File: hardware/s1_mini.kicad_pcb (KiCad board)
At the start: 2 copper layers, 31 x 54.4 mm, 12 parts, among them P1 USB_Edge, U1 AP2114H, U2 SM220UF1, U3 Wemos_D1_Mini

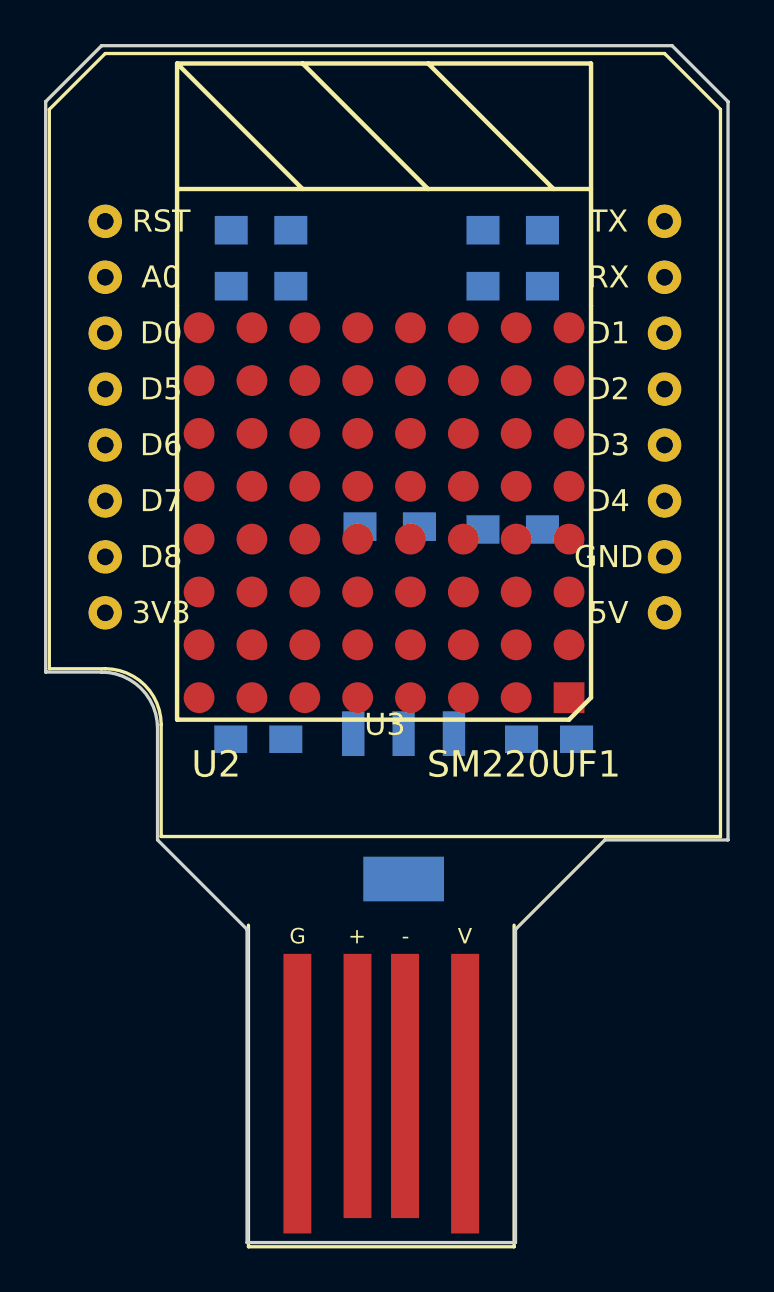
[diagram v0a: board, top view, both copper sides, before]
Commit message: Clean up part placements.
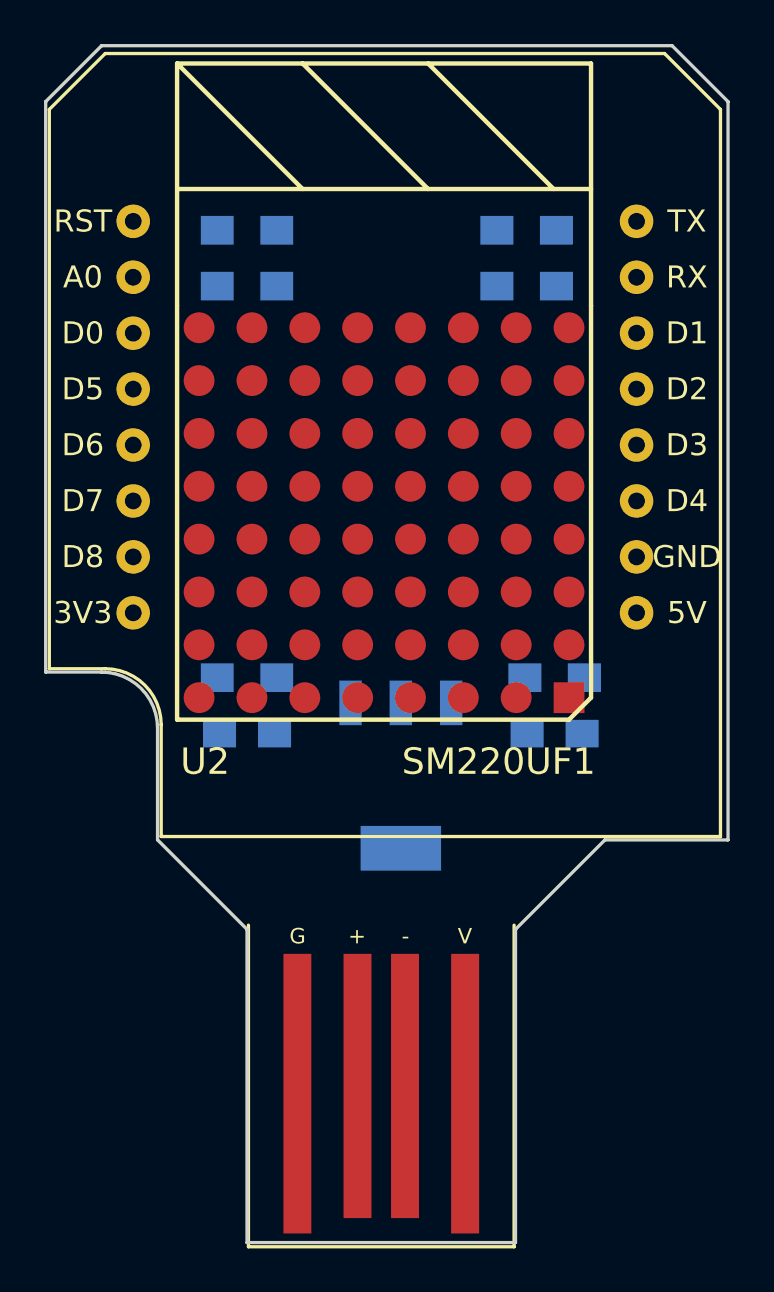
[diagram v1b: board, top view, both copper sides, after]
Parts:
- moved R6 13.8 mm to (142.2, 115.6)
- moved R5 10.2 mm to (156.2, 115.6)
- moved U1 1.40 mm to (149.2, 120.0)
- moved R1 0.63 mm to (142.2, 95.2)
- moved R2 0.63 mm to (154.9, 97.8)
- moved R3 0.63 mm to (142.2, 97.8)
- moved R4 0.63 mm to (154.9, 95.2)
- moved C2 0.57 mm to (142.2, 118.1)
- moved C1 0.36 mm to (156.2, 118.1)
